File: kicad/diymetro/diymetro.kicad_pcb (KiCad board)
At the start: 2 copper layers, 100 x 75 mm, 47 parts, among them J1 Conn_02x08_Top_Bottom, J10 ReverseSwitch, J11 Conn_01x04, J12 +5V, J2 CLKGATE_Pots, J3 Gate_Pots, J4 CV_Pots, J5 CLKOUT, J6 GATEOUT, J7 CVOUT, J8 LEDs, J9 Conn_01x04, U1 74HC4051, U2 74HC4051, U3 74LS594, U4 74LS165

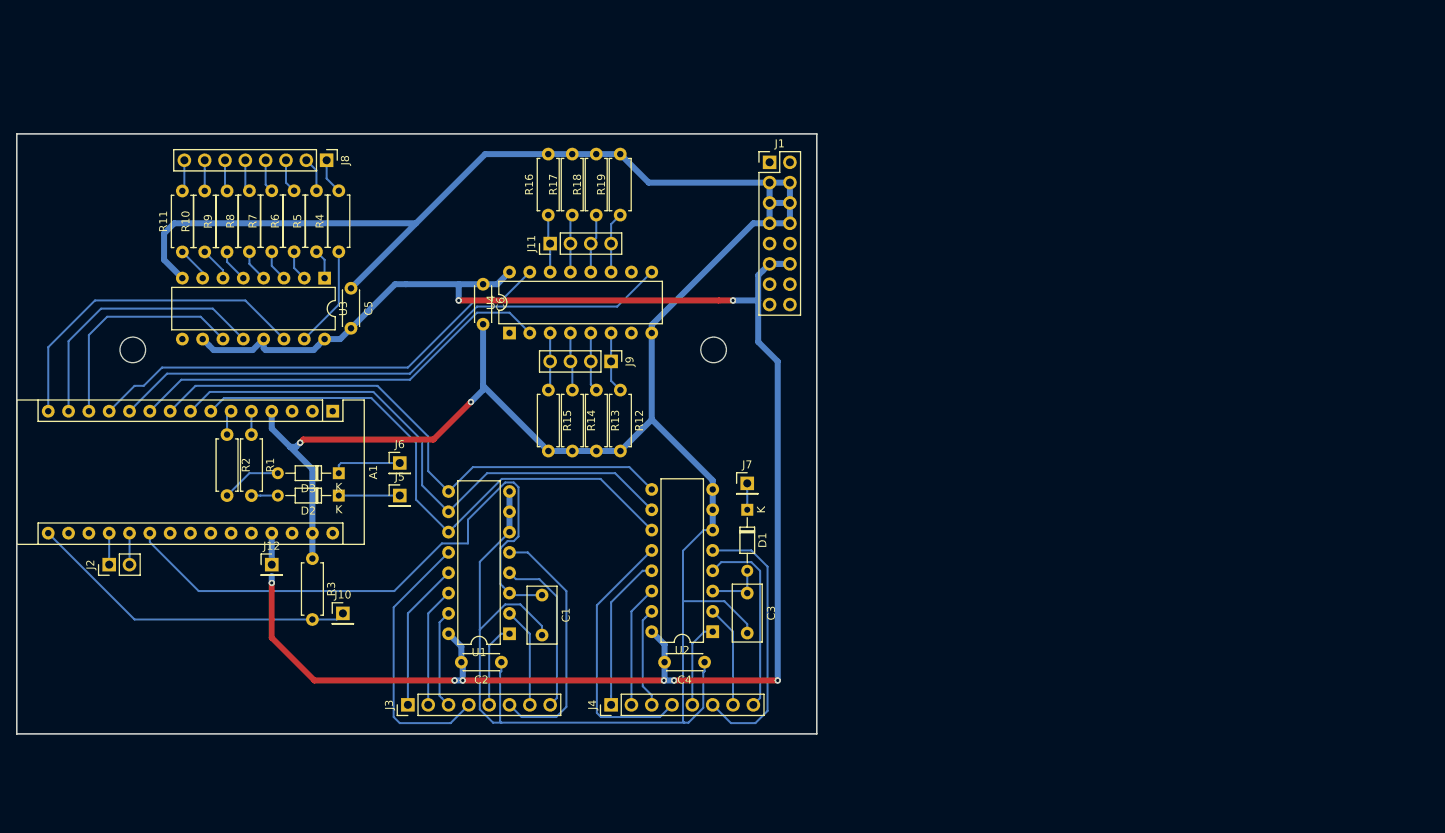
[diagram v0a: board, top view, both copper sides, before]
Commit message: New schematics and boards.
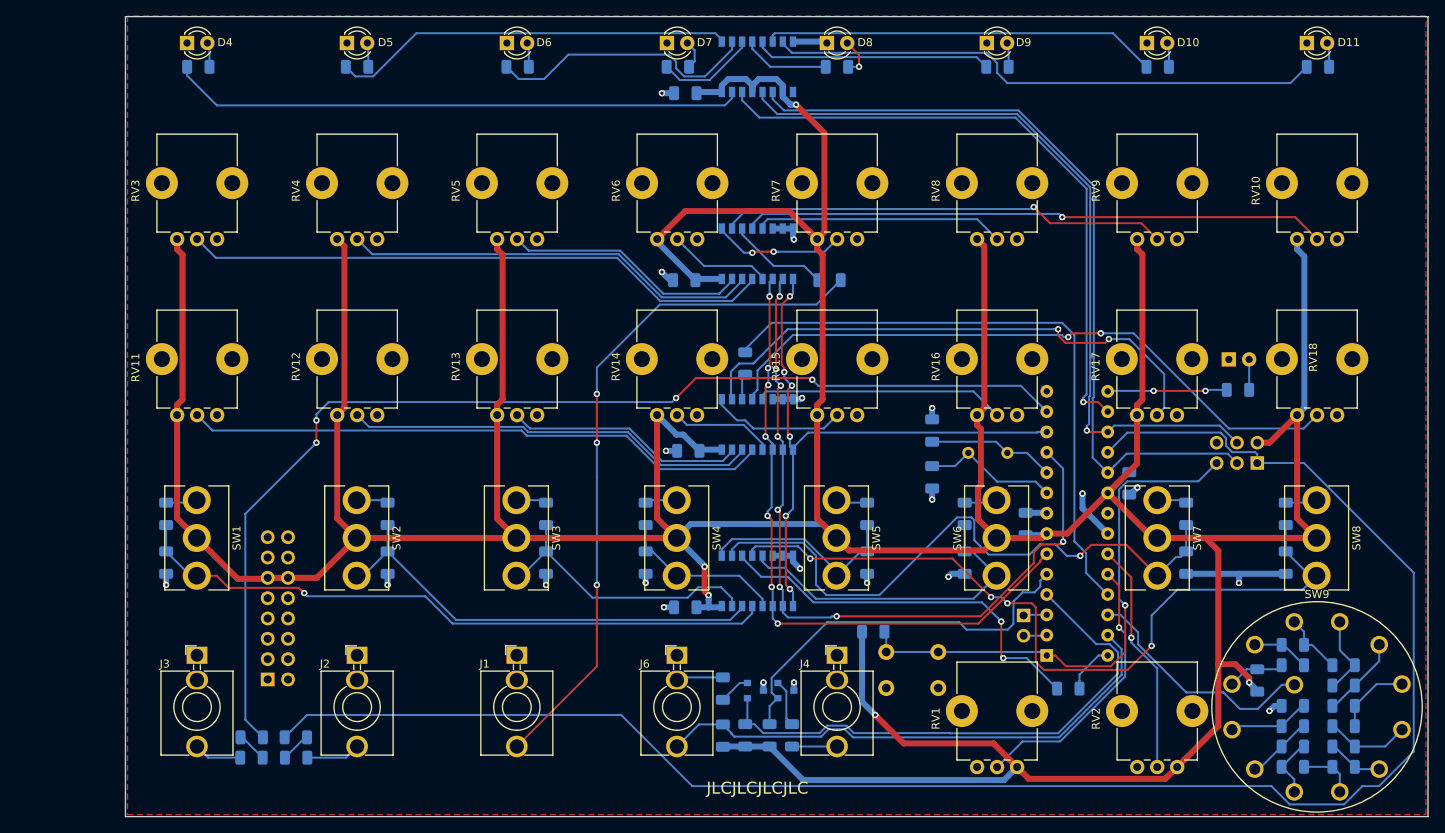
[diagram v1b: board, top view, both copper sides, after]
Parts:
- removed A1: Arduino_Nano_v3.x, Module:Arduino_Nano
- removed J10: ReverseSwitch, Connector_PinHeader_2.54mm:PinHeader_1x01_P2.54mm_Vertical
- removed J11, J9: Conn_01x04, Connector_PinHeader_2.54mm:PinHeader_1x04_P2.54mm_Vertical
- removed J12: +5V, Connector_PinHeader_2.54mm:PinHeader_1x01_P2.54mm_Vertical
- removed REF** (x2): MountingHole_3.2mm_M3, MountingHole:MountingHole_3.2mm_M3
- added C7: 100n, Capacitor_SMD:C_1206_3216Metric, B.Cu at (197.4, 97.3)
- added C8: 100n, Capacitor_SMD:C_1206_3216Metric, B.Cu at (184.4, 102.4)
- added D10: LED, LED_THT:LED_D3.0mm, F.Cu at (199.6, 42.2)
- added D11: LED, LED_THT:LED_D3.0mm, F.Cu at (219.6, 42.2)
- added D12: D, Diode_SMD:D_1206_3216Metric, B.Cu at (159.9, 71.9)
- added D13: D, Diode_SMD:D_1206_3216Metric, B.Cu at (149.4, 82.3)
- added D14: LED, LED_THT:LED_D3.0mm, B.Cu at (209.8, 81.8)
- added D4: LED, LED_THT:LED_D3.0mm, F.Cu at (79.6, 42.2)
- added D5: LED, LED_THT:LED_D3.0mm, F.Cu at (99.6, 42.2)
- added D6: LED, LED_THT:LED_D3.0mm, F.Cu at (119.6, 42.2)
- added D7: LED, LED_THT:LED_D3.0mm, F.Cu at (139.6, 42.2)
- added D8: LED, LED_THT:LED_D3.0mm, F.Cu at (159.6, 42.2)
- added D9: LED, LED_THT:LED_D3.0mm, F.Cu at (179.6, 42.2)
- added Q1: PN2222A, Package_TO_SOT_SMD:SOT-23, B.Cu at (154.4, 123.2)
- added Q2: PN2222A, Package_TO_SOT_SMD:SOT-23, B.Cu at (150.6, 123.2)
- added R20: 1K, Resistor_SMD:R_1206_3216Metric, B.Cu at (204.5, 101.1)
- added R21: 1K, Resistor_SMD:R_1206_3216Metric, B.Cu at (204.5, 107.2)
- added R22: 1K, Resistor_SMD:R_1206_3216Metric, B.Cu at (216.9, 101.1)
- added R23: 1K, Resistor_SMD:R_1206_3216Metric, B.Cu at (216.9, 107.2)
- added R24: 220, Resistor_SMD:R_1206_3216Metric, B.Cu at (81.0, 45.2)
- added R25: 220, Resistor_SMD:R_1206_3216Metric, B.Cu at (100.8, 45.2)
- added R26: 220, Resistor_SMD:R_1206_3216Metric, B.Cu at (120.9, 45.2)
- added R27: 220, Resistor_SMD:R_1206_3216Metric, B.Cu at (140.9, 45.2)
- added R28: 220, Resistor_SMD:R_1206_3216Metric, B.Cu at (160.8, 45.2)
- added R29: 220, Resistor_SMD:R_1206_3216Metric, B.Cu at (180.9, 45.2)
- added R30: 220, Resistor_SMD:R_1206_3216Metric, B.Cu at (200.9, 45.2)
- added R31: 220, Resistor_SMD:R_1206_3216Metric, B.Cu at (220.9, 45.2)
- added R32: 1K, Resistor_SMD:R_1206_3216Metric, B.Cu at (213.4, 121.9)
- added R33: 1K, Resistor_SMD:R_1206_3216Metric, B.Cu at (217.8, 120.0)
- added R34: 1K, Resistor_SMD:R_1206_3216Metric, B.Cu at (217.8, 117.5)
- added R35: 1K, Resistor_SMD:R_1206_3216Metric, B.Cu at (224.2, 120.0)
- added R36: 1K, Resistor_SMD:R_1206_3216Metric, B.Cu at (224.2, 122.6)
- added R37: 1K, Resistor_SMD:R_1206_3216Metric, B.Cu at (224.2, 125.1)
- added R38: 1K, Resistor_SMD:R_1206_3216Metric, B.Cu at (224.2, 127.6)
- added R39: 1K, Resistor_SMD:R_1206_3216Metric, B.Cu at (224.2, 130.2)
- added R40: 1K, Resistor_SMD:R_1206_3216Metric, B.Cu at (224.2, 132.7)
- added R41: 1K, Resistor_SMD:R_1206_3216Metric, B.Cu at (217.8, 132.7)
- added R42: 1K, Resistor_SMD:R_1206_3216Metric, B.Cu at (217.8, 130.2)
- added R43: 1K, Resistor_SMD:R_1206_3216Metric, B.Cu at (217.8, 127.6)
- added R44: 1K, Resistor_SMD:R_1206_3216Metric, B.Cu at (217.8, 125.1)
- added R45: 10k, Resistor_SMD:R_1206_3216Metric, B.Cu at (165.4, 115.8)
- added R46: 1K, Resistor_SMD:R_1206_3216Metric, B.Cu at (210.9, 85.6)
- added RV1: R_POT, Potentiometer_THT:Potentiometer_Alps_RK09K_Single_Vertical, F.Cu at (183.3, 132.7)
- added RV10: R_POT, Potentiometer_THT:Potentiometer_Alps_RK09K_Single_Vertical, F.Cu at (223.3, 66.8)
- added RV11: R_POT, Potentiometer_THT:Potentiometer_Alps_RK09K_Single_Vertical, F.Cu at (83.3, 88.7)
- added RV12: R_POT, Potentiometer_THT:Potentiometer_Alps_RK09K_Single_Vertical, F.Cu at (103.4, 88.7)
- added RV13: R_POT, Potentiometer_THT:Potentiometer_Alps_RK09K_Single_Vertical, F.Cu at (123.3, 88.7)
- added RV14: R_POT, Potentiometer_THT:Potentiometer_Alps_RK09K_Single_Vertical, F.Cu at (143.3, 88.7)
- added RV15: R_POT, Potentiometer_THT:Potentiometer_Alps_RK09K_Single_Vertical, F.Cu at (163.3, 88.7)
- added RV16: R_POT, Potentiometer_THT:Potentiometer_Alps_RK09K_Single_Vertical, F.Cu at (183.3, 88.7)
- added RV17: R_POT, Potentiometer_THT:Potentiometer_Alps_RK09K_Single_Vertical, F.Cu at (203.3, 88.7)
- added RV18: R_POT, Potentiometer_THT:Potentiometer_Alps_RK09K_Single_Vertical, F.Cu at (223.3, 88.7)
- added RV2: R_POT, Potentiometer_THT:Potentiometer_Alps_RK09K_Single_Vertical, F.Cu at (203.4, 132.7)
- added RV3: R_POT, Potentiometer_THT:Potentiometer_Alps_RK09K_Single_Vertical, F.Cu at (83.3, 66.8)
- added RV4: R_POT, Potentiometer_THT:Potentiometer_Alps_RK09K_Single_Vertical, F.Cu at (103.4, 66.8)
- added RV5: R_POT, Potentiometer_THT:Potentiometer_Alps_RK09K_Single_Vertical, F.Cu at (123.3, 66.8)
- added RV6: R_POT, Potentiometer_THT:Potentiometer_Alps_RK09K_Single_Vertical, F.Cu at (143.4, 66.8)
- added RV7: R_POT, Potentiometer_THT:Potentiometer_Alps_RK09K_Single_Vertical, F.Cu at (163.3, 66.8)
- added RV8: R_POT, Potentiometer_THT:Potentiometer_Alps_RK09K_Single_Vertical, F.Cu at (183.3, 66.8)
- added RV9: R_POT, Potentiometer_THT:Potentiometer_Alps_RK09K_Single_Vertical, F.Cu at (203.4, 66.8)
- added SW1: SW_SPDT_MSM, Tomarus:SPDT_Switch_4.72mm, F.Cu at (80.8, 104.1)
- added SW10: SW_Push, Button_Switch_THT:SW_PUSH_6mm, B.Cu at (173.5, 118.4)
- added SW2: SW_SPDT_MSM, Tomarus:SPDT_Switch_4.72mm, F.Cu at (100.8, 104.1)
- added SW3: SW_SPDT_MSM, Tomarus:SPDT_Switch_4.72mm, F.Cu at (120.8, 104.1)
- added SW4: SW_SPDT_MSM, Tomarus:SPDT_Switch_4.72mm, F.Cu at (140.8, 104.1)
- added SW5: SW_SPDT_MSM, Tomarus:SPDT_Switch_4.72mm, F.Cu at (160.8, 104.1)
- added SW6: SW_SPDT_MSM, Tomarus:SPDT_Switch_4.72mm, F.Cu at (180.8, 104.1)
- added SW7: SW_SPDT_MSM, Tomarus:SPDT_Switch_4.72mm, F.Cu at (200.9, 104.1)
- added SW8: SW_SPDT_MSM, Tomarus:SPDT_Switch_4.72mm, F.Cu at (220.8, 104.1)
- added SW9: SW_Rotary12, Tomarus:SR2612F_RotarySwitch, F.Cu at (220.8, 125.2)
- added U5: ATmega328P-PU, Package_DIP:DIP-28_W7.62mm, B.Cu at (187.0, 118.8)
- added Y1: Crystal, Crystal:Crystal_HC49-4H_Vertical, B.Cu at (182.1, 93.5)
- C1, C3: value 220n -> 100n; footprint Capacitor_THT:C_Rect_L7.0mm_W3.5mm_P5.00mm -> Capacitor_SMD:C_1206_3216Metric; moved to B.Cu
- C2, C4: footprint Capacitor_THT:C_Disc_D4.3mm_W1.9mm_P5.00mm -> Capacitor_SMD:C_1206_3216Metric; moved to B.Cu
- C5, C6: value 100n -> 22p; footprint Capacitor_THT:C_Disc_D4.3mm_W1.9mm_P5.00mm -> Capacitor_SMD:C_1206_3216Metric; moved to B.Cu
- D1, D2, D3: footprint Diode_THT:D_DO-34_SOD68_P7.62mm_Horizontal -> Diode_SMD:D_1206_3216Metric; moved to B.Cu
- J1: value Conn_02x08_Top_Bottom -> AudioJack2_SwitchT; footprint Connector_PinHeader_2.54mm:PinHeader_2x08_P2.54mm_Vertical -> Connector_Audio:Jack_3.5mm_QingPu_WQP-PJ398SM_Vertical_CircularHoles
- J2: value CLKGATE_Pots -> AudioJack2_SwitchT; footprint Connector_PinHeader_2.54mm:PinHeader_1x02_P2.54mm_Vertical -> Connector_Audio:Jack_3.5mm_QingPu_WQP-PJ398SM_Vertical_CircularHoles
- J3: value Gate_Pots -> AudioJack2_SwitchT; footprint Connector_PinHeader_2.54mm:PinHeader_1x08_P2.54mm_Vertical -> Connector_Audio:Jack_3.5mm_QingPu_WQP-PJ398SM_Vertical_CircularHoles
- J4: value CV_Pots -> AudioJack2_SwitchT; footprint Connector_PinHeader_2.54mm:PinHeader_1x08_P2.54mm_Vertical -> Connector_Audio:Jack_3.5mm_QingPu_WQP-PJ398SM_Vertical_CircularHoles
- J5: value CLKOUT -> Conn_02x08_Top_Bottom; footprint Connector_PinHeader_2.54mm:PinHeader_1x01_P2.54mm_Vertical -> Connector_IDC:IDC-Header_2x08_P2.54mm_Vertical; moved to B.Cu
- J6: value GATEOUT -> AudioJack2_SwitchT; footprint Connector_PinHeader_2.54mm:PinHeader_1x01_P2.54mm_Vertical -> Connector_Audio:Jack_3.5mm_QingPu_WQP-PJ398SM_Vertical_CircularHoles
- J7: value CVOUT -> ICSP; footprint Connector_PinHeader_2.54mm:PinHeader_1x01_P2.54mm_Vertical -> Connector_PinHeader_2.54mm:PinHeader_2x03_P2.54mm_Vertical; moved to B.Cu
- J8: value LEDs -> SER; footprint Connector_PinHeader_2.54mm:PinHeader_1x08_P2.54mm_Vertical -> Connector_PinHeader_2.54mm:PinHeader_1x02_P2.54mm_Vertical; moved to B.Cu
- R1, R2, R3: footprint Resistor_THT:R_Axial_DIN0207_L6.3mm_D2.5mm_P7.62mm_Horizontal -> Resistor_SMD:R_1206_3216Metric; moved to B.Cu
- R10, R11, R8, R9: value 220 -> 1K; footprint Resistor_THT:R_Axial_DIN0207_L6.3mm_D2.5mm_P7.62mm_Horizontal -> Resistor_SMD:R_1206_3216Metric; moved to B.Cu
- R12, R13, R14, R15, R16, R17, R18, R19: value 10K -> 1K; footprint Resistor_THT:R_Axial_DIN0207_L6.3mm_D2.5mm_P7.62mm_Horizontal -> Resistor_SMD:R_1206_3216Metric; moved to B.Cu
- R4, R7: value 220 -> 100K; footprint Resistor_THT:R_Axial_DIN0207_L6.3mm_D2.5mm_P7.62mm_Horizontal -> Resistor_SMD:R_1206_3216Metric; moved to B.Cu
- R5: value 220 -> 10K; footprint Resistor_THT:R_Axial_DIN0207_L6.3mm_D2.5mm_P7.62mm_Horizontal -> Resistor_SMD:R_1206_3216Metric; moved to B.Cu
- R6: value 220 -> 1M; footprint Resistor_THT:R_Axial_DIN0207_L6.3mm_D2.5mm_P7.62mm_Horizontal -> Resistor_SMD:R_1206_3216Metric; moved to B.Cu
- U1: footprint Package_DIP:DIP-16_W7.62mm -> Package_SO:SOP-16_4.4x10.4mm_P1.27mm; moved to B.Cu
- U2: value 74HC4051 -> 74LS595; footprint Package_DIP:DIP-16_W7.62mm -> Package_SO:SOP-16_4.4x10.4mm_P1.27mm; moved to B.Cu
- U3: value 74LS594 -> 74HC4051; footprint Package_DIP:DIP-16_W7.62mm -> Package_SO:SOP-16_4.4x10.4mm_P1.27mm; moved to B.Cu
- U4: value 74LS165 -> 74HC4051; footprint Package_DIP:DIP-16_W7.62mm -> Package_SO:SOP-16_4.4x10.4mm_P1.27mm; moved to B.Cu
- moved J8 104.1 mm to (184.2, 113.8), turned to 180 degrees
- moved D3 95.1 mm to (189.7, 122.9)
- moved R4 82.8 mm to (155.2, 128.8), turned to 270 degrees
- moved R6 80.8 mm to (146.6, 128.8)
- moved R5 80.8 mm to (149.4, 128.8)
- moved R7 78.5 mm to (146.6, 122.9)
- moved C5 74.8 mm to (172.7, 90.7)
- moved C2 74.7 mm to (141.9, 48.5), turned to 0 degrees
- moved U2 70.8 mm to (150.9, 45.2), turned to 270 degrees
- moved D1 69.3 mm to (87.6, 131.6), turned to 0 degrees
- moved J1 69.2 mm to (120.8, 118.8)
- moved J7 63.8 mm to (213.4, 94.7), turned to 90 degrees
- moved R3 61.3 mm to (152.4, 128.8), turned to 90 degrees
- moved R19 61.2 mm to (176.8, 107.2)
- moved C6 61.1 mm to (172.7, 96.5), turned to 90 degrees
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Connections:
- C1 pad 1: Net-(A1-Pad21) -> GND
- C1 pad 2: GND -> +5V
- C3 pad 1: Net-(C3-Pad1) -> GND
- C3 pad 2: GND -> +5V
- C5 pad 2: +5V -> Net-(C5-Pad2)
- C6 pad 1: +5V -> GND
- C6 pad 2: GND -> Net-(C6-Pad2)
- D1 pad 1: Net-(D1-Pad1) -> /AP_CLK_OUT
- D1 pad 2: Net-(C3-Pad1) -> Net-(D1-Pad2)
- D2 pad 1: Net-(D2-Pad1) -> /AP_GATE_OUT
- D3 pad 1: Net-(D3-Pad1) -> SA
- J5 pad 1: Net-(D2-Pad1) -> Net-(J5-Pad1)
- J7 pad 1: Net-(D1-Pad1) -> /ICSP_MISO
- R1 pad 2: Net-(D2-Pad2) -> Net-(D1-Pad2)
- R10 pad 1: Net-(R10-Pad1) -> /Switches/SW1
- R10 pad 2: Net-(J8-Pad7) -> Net-(R10-Pad2)
- R11 pad 1: Net-(R11-Pad1) -> GND
- R11 pad 2: Net-(J8-Pad8) -> /Switches/SW1
- R12 pad 1: Net-(J9-Pad1) -> /Switches/SW2
- R12 pad 2: GND -> Net-(R12-Pad2)
- R13 pad 1: Net-(J9-Pad2) -> GND
- R13 pad 2: GND -> /Switches/SW2
- R14 pad 1: Net-(J9-Pad3) -> /Switches/SW3
- R14 pad 2: GND -> Net-(R14-Pad2)
- R15 pad 1: Net-(J9-Pad4) -> GND
- R15 pad 2: GND -> /Switches/SW3
- R16 pad 1: Net-(J11-Pad1) -> /Switches/SW4
- R16 pad 2: GND -> Net-(R16-Pad2)
- R17 pad 1: Net-(J11-Pad2) -> GND
- R17 pad 2: GND -> /Switches/SW4
- R18 pad 1: Net-(J11-Pad3) -> /Switches/SW5
- R18 pad 2: GND -> Net-(R18-Pad2)
- R19 pad 1: Net-(J11-Pad4) -> GND
- R19 pad 2: GND -> /Switches/SW5
- R2 pad 1: Net-(A1-Pad6) -> /ICSP_MISO
- R2 pad 2: Net-(D3-Pad2) -> Net-(D2-Pad2)
- R3 pad 1: GND -> +5V
- R3 pad 2: Net-(A1-Pad16) -> /AP_RST_IN
- R4 pad 1: Net-(R4-Pad1) -> Net-(Q1-Pad2)
- R4 pad 2: Net-(J8-Pad1) -> Net-(J4-PadT)
- R5 pad 1: Net-(R5-Pad1) -> +5V
- R5 pad 2: Net-(J8-Pad2) -> /AP_CLK_IN
- R6 pad 1: Net-(R6-Pad1) -> +5V
- R6 pad 2: Net-(J8-Pad3) -> CINSW
- R7 pad 1: Net-(R7-Pad1) -> Net-(Q2-Pad2)
- R7 pad 2: Net-(J8-Pad4) -> Net-(J6-PadTN)
- R8 pad 1: Net-(R8-Pad1) -> /Switches/SW0
- R8 pad 2: Net-(J8-Pad5) -> Net-(R8-Pad2)
- R9 pad 1: Net-(R9-Pad1) -> GND
- R9 pad 2: Net-(J8-Pad6) -> /Switches/SW0
- U1 pad 1: Net-(J3-Pad5) -> /Switches/SW4
- U1 pad 12: Net-(J3-Pad4) -> /Switches/SW3
- U1 pad 13: Net-(J3-Pad1) -> /Switches/SW0
- U1 pad 14: Net-(J3-Pad2) -> /Switches/SW1
- U1 pad 15: Net-(J3-Pad3) -> /Switches/SW2
- U1 pad 2: Net-(J3-Pad7) -> /Switches/SW6
- U1 pad 3: Net-(A1-Pad21) -> Net-(D3-Pad2)
- U1 pad 4: Net-(J3-Pad8) -> /Switches/SW7
- U1 pad 5: Net-(J3-Pad6) -> /Switches/SW5
- U2 pad 1: Net-(J4-Pad5) -> Net-(R25-Pad1)
- U2 pad 10: S1 -> +5V
- U2 pad 11: S0 -> SCLK
- U2 pad 12: Net-(J4-Pad4) -> RCLK
- U2 pad 13: Net-(J4-Pad1) -> +5V
- U2 pad 14: Net-(J4-Pad2) -> SER
- U2 pad 15: Net-(J4-Pad3) -> Net-(R24-Pad1)
- U2 pad 2: Net-(J4-Pad7) -> Net-(R26-Pad1)
- U2 pad 3: Net-(C3-Pad1) -> Net-(R27-Pad1)
- U2 pad 4: Net-(J4-Pad8) -> Net-(R28-Pad1)
- U2 pad 5: Net-(J4-Pad6) -> Net-(R29-Pad1)
- U2 pad 6: GND -> Net-(R30-Pad1)
- U2 pad 7: GND -> Net-(R31-Pad1)
- U2 pad 9: S2 -> Net-(U2-Pad9)
- U3 pad 1: Net-(R5-Pad1) -> /CV Pots/A4
- U3 pad 10: +5V -> S1
- U3 pad 11: SCLK -> S0
- U3 pad 12: RCLK -> /CV Pots/A3
- U3 pad 13: +5V -> /CV Pots/A0
- U3 pad 14: SER -> /CV Pots/A1
- U3 pad 15: Net-(R4-Pad1) -> /CV Pots/A2
- U3 pad 2: Net-(R6-Pad1) -> /CV Pots/A6
- U3 pad 3: Net-(R7-Pad1) -> Net-(D12-Pad2)
- U3 pad 4: Net-(R8-Pad1) -> /CV Pots/A7
- U3 pad 5: Net-(R9-Pad1) -> /CV Pots/A5
- U3 pad 6: Net-(R10-Pad1) -> GND
- U3 pad 7: Net-(R11-Pad1) -> GND
- U3 pad 9: Net-(U3-Pad9) -> S2
- U4 pad 1: Net-(U4-Pad1) -> /Gate Pots/GA4
- U4 pad 10: Net-(U4-Pad10) -> S1
- U4 pad 11: Net-(J11-Pad4) -> S0
- U4 pad 12: Net-(J11-Pad3) -> /Gate Pots/GA3
- U4 pad 13: Net-(J11-Pad2) -> /Gate Pots/GA0
- U4 pad 14: Net-(J11-Pad1) -> /Gate Pots/GA1
- U4 pad 15: CE -> /Gate Pots/GA2
- U4 pad 2: CP -> /Gate Pots/GA6
- U4 pad 3: Net-(J9-Pad4) -> Net-(D13-Pad2)
- U4 pad 4: Net-(J9-Pad3) -> /Gate Pots/GA7
- U4 pad 5: Net-(J9-Pad2) -> /Gate Pots/GA5
- U4 pad 6: Net-(J9-Pad1) -> GND
- U4 pad 7: Net-(U4-Pad7) -> GND
- U4 pad 9: QH -> S2
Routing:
- net +5V: track 229.1 -> 678.9 mm, vias 8 -> 5
- net GND: track 367.5 -> 61.4 mm, vias 2 -> 22
- net /ICSP_MISO: track 0.00 -> 219.7 mm
- net Net-(R1-Pad1): track 2.92 -> 139.9 mm, vias 0 -> 4
- net /Switches/SW7: track 0.00 -> 97.4 mm, vias 0 -> 4
- net PIN_CVOUT: track 0.00 -> 86.5 mm, vias 0 -> 3
- net /Switches/SW0: track 0.00 -> 81.7 mm, vias 0 -> 1
- net /Gate Pots/GA7: track 0.00 -> 81.6 mm, vias 0 -> 2
- net /Switches/SW6: track 0.00 -> 78.0 mm, vias 0 -> 1
- net PIN_GATEOUT: track 0.00 -> 77.7 mm
- net Net-(A1-Pad21): track 76.6 -> 0.00 mm
- net /CV Pots/A0: track 0.00 -> 73.9 mm
- net /Gate Pots/GA0: track 0.00 -> 73.4 mm
- net /CV Pots/A7: track 0.00 -> 73.0 mm, vias 0 -> 1
- net QH: track 72.5 -> 0.00 mm
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- added copper zone on F.Cu, net GND
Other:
- board size 100 x 75 mm -> 162.8 x 100 mm
- board text added: "."
- board text added: "ICSP"
- board text added: "JLCJLCJLCJLC"
- board text added: "R32-44"
- board text added: "RED STRIPE"
- board text added: "SER"
- board text added: "Tomarus Sequencer v1.0 github.com/tomarus/diymetro Inspired by Ryk & Intellijel"
